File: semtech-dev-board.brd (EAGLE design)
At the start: 73.4 x 82.5 mm, 62 parts, among them Q1 BSS123, Q2 32MHz, U1 SEMTECH_SX1236, U2 QUALCOMM-TDK_B3588, U3 MIC5219 3.3V, U4 QUALCOMM-TDK_B3710

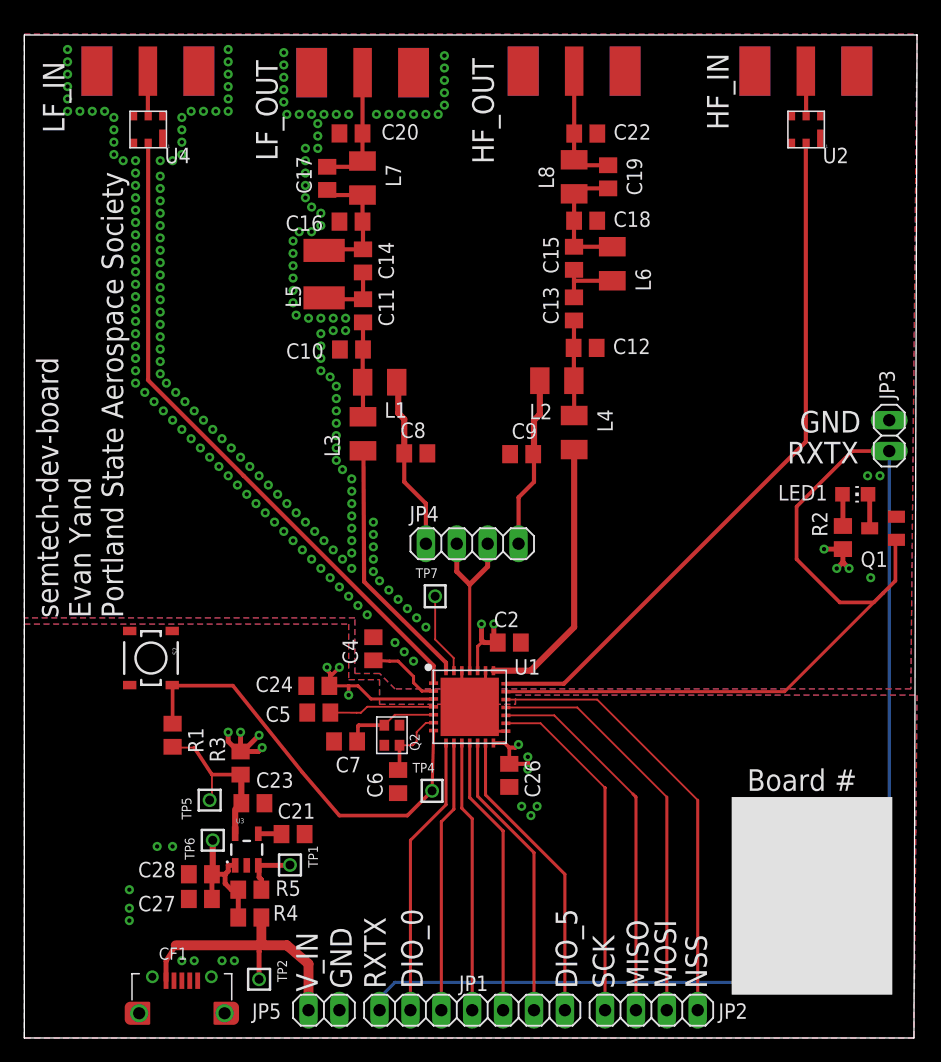
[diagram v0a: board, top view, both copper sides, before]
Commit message: Tuesday D/R
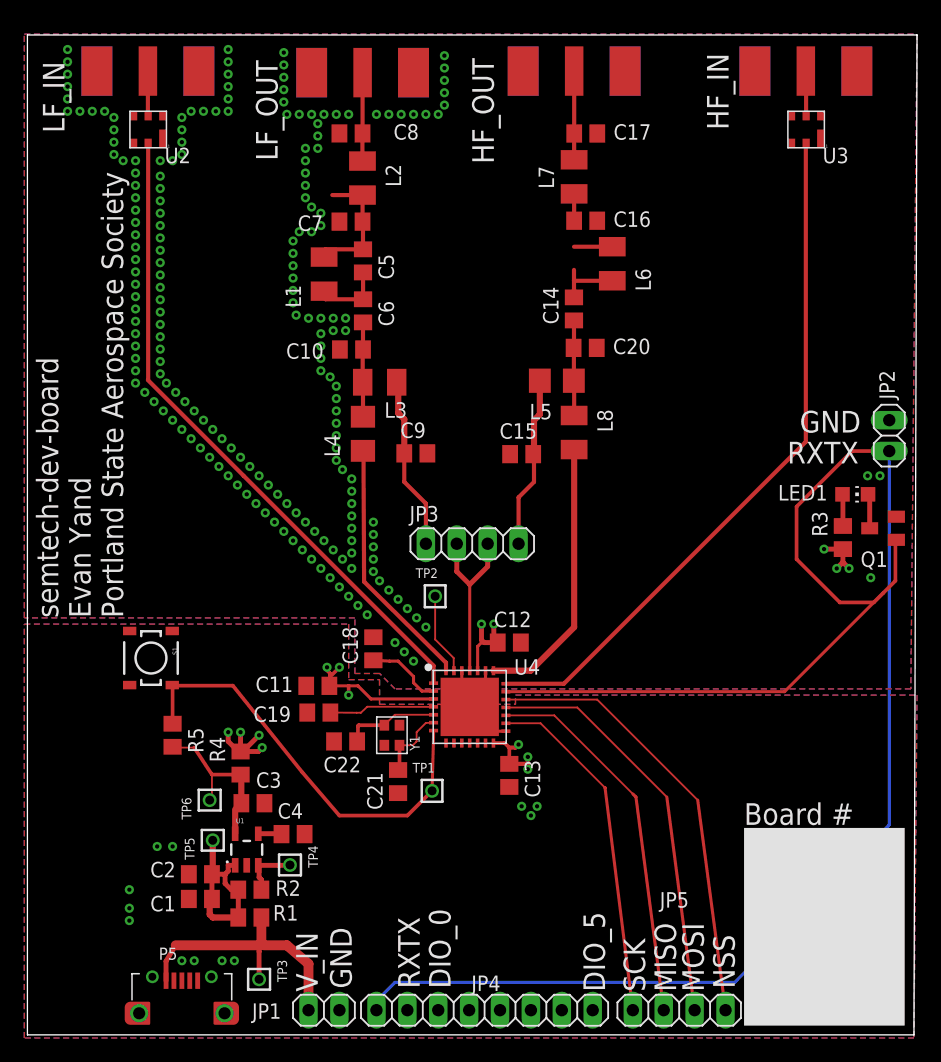
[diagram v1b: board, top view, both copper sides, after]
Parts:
- removed C24, C26, C28: 100nF, rcl:C0805
- removed TP7: TEST-POINT, low-gain-radio:2MM-TEST-POINT
- added TP3: TEST-POINT, low-gain-radio:2MM-TEST-POINT
- C11: value 22pF -> 100nF
- C12: value 4.7pF -> 100nF
- C13: value 8.2pF -> 100nF
- C14: value 2.7pF -> 8.2pF
- C15: value ?? -> 10nF
- C16: value 15pF -> 6.8pF
- C17: value ?? -> 5.6pF
- C18: value 6.8pF -> 100nF
- C19: value ?? -> 100nF
- C20: value 8.2pF -> 4.7pF
- C21: value 470pF -> 15pF
- C22: value 5.6pF -> 15pF
- C4: value 100nF -> 470pF
- C5: value 100nF -> 2.7pF
- C6: value 6pF -> 22pF
- C7: value 6pF -> 15pF
- C8: value 10nF -> 8.2pF
- JP1: device pinhead:1X07 -> pinhead:1X02
- JP2: device pinhead:1X04 -> pinhead:1X02
- JP3, JP5: device pinhead:1X02 -> pinhead:1X04
- JP4: device pinhead:1X04 -> pinhead:1X08
- L1: value 33nH -> 12nH; device rcl:L3230M -> rcl:L3225M
- L2: value 33nH -> 10nH; device rcl:L3230M -> rcl:L3225M
- L3: value 10nH -> 33nH; device rcl:L3230M -> rcl:L3225M
- L4: value 3.9nH -> 10nH; device rcl:L3230M -> rcl:L3225P
- L5: value 12nH -> 33nH; device rcl:L1812 -> rcl:L3225P
- L6: device rcl:L3230M -> rcl:L3225M
- L7: value 10nH -> 6.8nH; device rcl:L3230M -> rcl:L3225M
- L8: value 6.8nH -> 3.9nH; device rcl:L3230M -> rcl:L3225M
- R1: value 1k -> 0
- R5: value 0 -> 1k
- U1: value SEMTECH_SX1236 -> MIC5219 3.3V; device low-gain-radio:QFN28 -> SparkFun-IC-Power:SOT23-5
- U2: value QUALCOMM-TDK_B3588 -> QUALCOMM-TDK_B3710
- U3: value MIC5219 3.3V -> QUALCOMM-TDK_B3588; device SparkFun-IC-Power:SOT23-5 -> low-gain-radio:DCC6C
- U4: value QUALCOMM-TDK_B3710 -> SEMTECH_SX1236; device low-gain-radio:DCC6C -> low-gain-radio:QFN28
- moved U3 77.1 mm to (65.5, 75.9), turned to 180 degrees
- moved R2 56.7 mm to (18.3, 11.9), turned to 180 degrees
- moved U4 56.6 mm to (33.0, 23.6), turned to 0 degrees
- moved U2 54.1 mm to (11.4, 75.9)
- moved C22 53.7 mm to (26.2, 24.1), turned to 180 degrees
- moved R3 52.9 mm to (67.1, 40.9)
- moved JP2 51.1 mm to (70.9, 49.3), turned to 90 degrees
- moved C19 50.1 mm to (24.0, 26.5), turned to 180 degrees
- moved C7 42.7 mm to (26.6, 66.9)
- moved C18 39.3 mm to (28.4, 31.8), turned to 90 degrees
- moved C6 38.8 mm to (27.6, 59.5), turned to 90 degrees
- moved C13 38.7 mm to (39.6, 21.3), turned to 270 degrees
- moved JP4 38.4 mm to (37.6, 2.03)
- moved C5 37.3 mm to (27.6, 63.6), turned to 90 degrees
- moved JP3 35.4 mm to (36.6, 40.4), turned to 0 degrees
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- renumbered C23 to C3, C27 to C1, CF1 to P5, Q2 to Y1, S2 to S1, U$1 to P1, U$2 to P2, U$3 to P3, U$4 to P4
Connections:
- removed net DIO0: JP1.2, U1.8
- removed net DIO1: JP1.3, U1.9
- removed net DIO2: JP1.4, U1.10
- removed net DIO3: JP1.5, U1.11
- removed net DIO4: JP1.6, U1.12
- removed net DIO5: JP1.7, U1.13
- new net N$2: JP4.8, U4.13
- new net N$4: JP4.7, U4.12
- new net N$6: JP4.6, U4.11
- new net N$7: JP4.5, U4.10
- new net N$8: JP4.4, U4.9
- new net N$9: JP4.3, U4.8
- net +3V3: now also R4.2, R5.2, TP6.1, U1.5; no longer R1.2, R3.2, TP5.1, U3.5
- net BP: now also C4.1, U1.4; no longer C21.1, U3.4
- net GND: now also C11.2, C13.2, C15.2, C17.2, C19.2, JP1.2, JP2.2, U1.2, U3.P$1, U3.P$3, U3.P$4, U3.P$6, U4.0, U4.15, U4.23, U4.26; no longer C24.2, C26.2, C28.2, C5.2, C6.2, JP3.2, JP5.2, U1.0, U1.15, U1.23, U1.26, U3.2, U4.P$1, U4.P$3, U4.P$4, U4.P$6
- net HFO_PA_HEAD: now also C15.1, JP3.4, L5.2; no longer C9.1, JP4.4, L2.2
- net LED+: now also R3.1; no longer R2.1
- net LFO_PA_HEAD: now also C9.1, JP3.1, L3.2; no longer C8.1, JP4.1, L1.2
- net N$1: now also R2.1, TP4.1, U1.3; no longer R5.1, TP1.1, U3.3
- net N$5: now also U2.P$5; no longer U4.P$5
- net PA_BOOST: now also TP2.1, U4.27; no longer TP7.1, U1.27
- net RFI_HF: now also U3.P$2, U4.21; no longer U1.21, U2.P$2
- net RFI_HF_ANT: now also U3.P$5; no longer U2.P$5
- net RFI_LF: now also U2.P$2, U4.1; no longer U1.1, U4.P$2
- net RFO_HF: now also L8.2, U4.22; no longer L4.2, U1.22
- net RFO_HF_1: now also C14.2; no longer C13.2, C15.1
- net RFO_HF_2: now also C16.1, L7.2; no longer C15.2, C18.1, C19.1, L8.2
- net RFO_HF_OUT: now also C17.1, L7.1; no longer C19.2, C22.1, L8.1
- net RFO_HF_PA: now also C14.1, C20.1, L5.1, L8.1; no longer C12.1, C13.1, L2.1, L4.1
- net RFO_LF: now also L4.1, U4.28; no longer L3.1, U1.28
- net RFO_LF_1: now also C5.1, C6.2, L1.2; no longer C11.2, C14.1, L5.2
- net RFO_LF_2: now also C5.2, C7.1, L1.1, L2.2; no longer C14.2, C16.1, C17.1, L5.1, L7.2
- net RFO_LF_OUT: now also C8.1, L2.1; no longer C17.2, C20.1, L7.1
- net RFO_LF_PA: now also C6.1, L3.1, L4.2; no longer C11.1, L1.1, L3.2
- net RXTX: now also JP2.1, JP4.2, U4.20; no longer JP1.1, JP3.1, U1.20
- net SPI_MISO: now also JP5.2, U4.17; no longer JP2.2, U1.17
- net SPI_MOSI: now also JP5.3, U4.18; no longer JP2.3, U1.18
- net SPI_NSS: now also JP5.4, U4.19; no longer JP2.4, U1.19
- net SPI_SCK: now also JP5.1, U4.16; no longer JP2.1, U1.16
- net SX1236_RST: now also JP4.1, R5.1, TP1.1, U4.7; no longer R1.1, TP4.1, U1.7
- net VBAT: now also C11.1, C12.1, C13.1, R3.2, R4.1, U4.14, U4.24, U4.3; no longer C2.1, C24.1, C26.1, R2.2, R3.1, U1.14, U1.24, U1.3
- net VREG_IN: now also C2.1, R1.2, R2.2, TP5.1, U1.1; no longer C28.1, R4.2, R5.2, TP6.1, U3.1
- net VR_ANA: now also C18.1, U4.2; no longer C4.1, U1.2
- net VR_DIG: now also C19.1, U4.4; no longer C5.1, U1.4
- net VR_PA: now also JP3.2, JP3.3, U4.25; no longer JP4.2, JP4.3, U1.25
- net V_IN: now also JP1.1, R1.1, TP3.1; no longer JP5.1, R4.1, TP2.1
- net XTALA: now also C22.1, U4.5; no longer C7.1, U1.5
- net XTALB: now also C21.1, U4.6; no longer C6.1, U1.6
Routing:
- net DIO5: track 24.7 -> 0.00 mm
- net DIO4: track 23.9 -> 0.00 mm
- net DIO0: track 23.2 -> 0.00 mm
- net DIO3: track 23.1 -> 0.00 mm
- net DIO1: track 22.4 -> 0.00 mm
- net DIO2: track 22.3 -> 0.00 mm
- net RFO_HF_2: track 10.5 -> 6.00 mm
- net VREG_IN: track 11.8 -> 15.6 mm
- net RFO_LF_OUT: track 10.4 -> 7.95 mm
- net RFO_HF_OUT: track 10.3 -> 7.93 mm
- net RXTX: track 141.6 -> 140.6 mm
- net RFO_LF_1: track 5.46 -> 5.97 mm
- added copper zone on layer 2, net GND
- added copper zone on layer 15, net VBAT
- removed copper zone on layer 2, net VBAT
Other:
- board size 73.4 x 82.5 mm -> 73.2 x 82.2 mm
